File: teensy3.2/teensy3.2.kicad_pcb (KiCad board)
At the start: 2 copper layers, 31 parts, among them J1 USB_B_Micro, J2 Conn_01x26, J3 Conn_01x26, SW1 Prog, U1 LP38691SD-3.3, U2 MKL02Z32VFG4, U3 MK20DX256VLH7, Y1 32.768 KHz, Y2 16 MHz

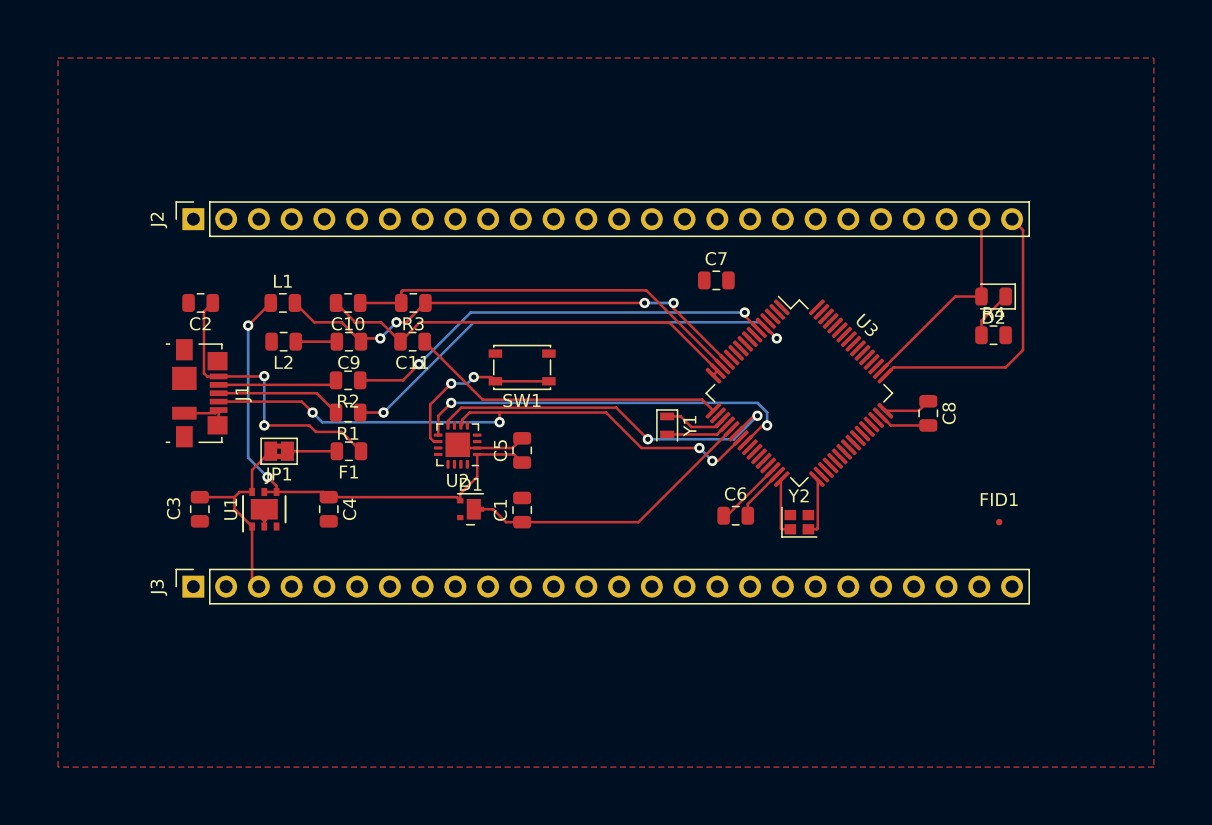
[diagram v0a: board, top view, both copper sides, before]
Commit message: fin ruteo pcb
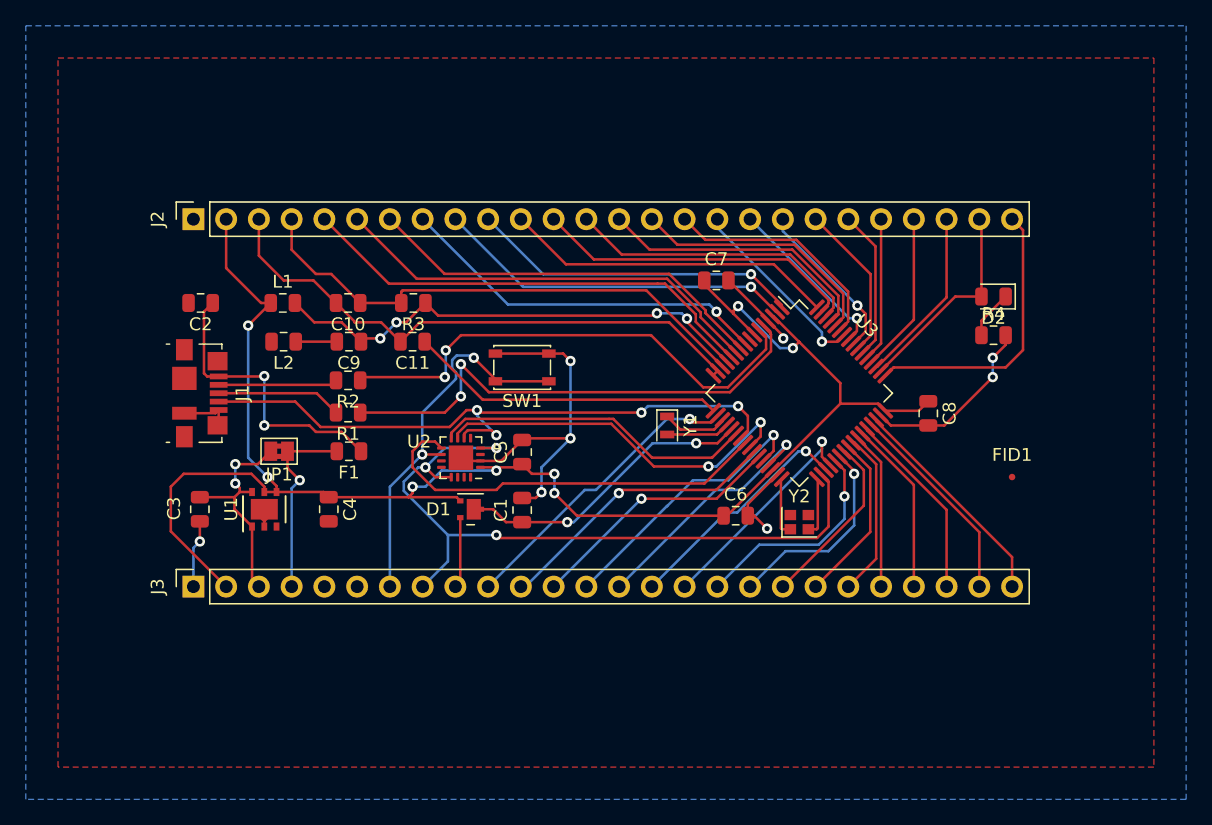
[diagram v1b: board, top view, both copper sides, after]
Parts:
- moved FID1 3.64 mm to (166.0, 99.5)
- moved U2 1.03 mm to (123.2, 98.0)
- moved C5 0.12 mm to (128.0, 97.6)
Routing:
- net +3V3: track 48.6 -> 129.7 mm, vias 2 -> 8
- net /RESET: track 0.00 -> 56.4 mm, vias 0 -> 3
- net GND: track 21.1 -> 67.6 mm, vias 0 -> 8
- net /J2_5: track 0.00 -> 37.1 mm
- net /J2_6: track 0.00 -> 33.9 mm
- net /J2_7: track 0.00 -> 31.5 mm
- net /PTA3: track 0.00 -> 29.3 mm, vias 0 -> 2
- net /J2_8: track 0.00 -> 29.2 mm, vias 0 -> 1
- net /J2_9: track 0.00 -> 27.9 mm, vias 0 -> 1
- net Net-(J2-Pad11): track 0.00 -> 25.8 mm
- net /J2_10: track 0.00 -> 25.7 mm, vias 0 -> 1
- net Net-(J2-Pad12): track 0.00 -> 25.1 mm
- net Net-(J3-Pad10): track 0.00 -> 23.6 mm, vias 0 -> 1
- net Net-(J2-Pad13): track 0.00 -> 23.4 mm
- net /J2_11: track 0.00 -> 22.4 mm, vias 0 -> 1
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- added copper zone on B.Cu, net GND
